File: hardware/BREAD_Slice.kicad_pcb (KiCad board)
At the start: 2 copper layers, 70 x 100 mm, 15 parts, among them J1 Conn_01x10_Female

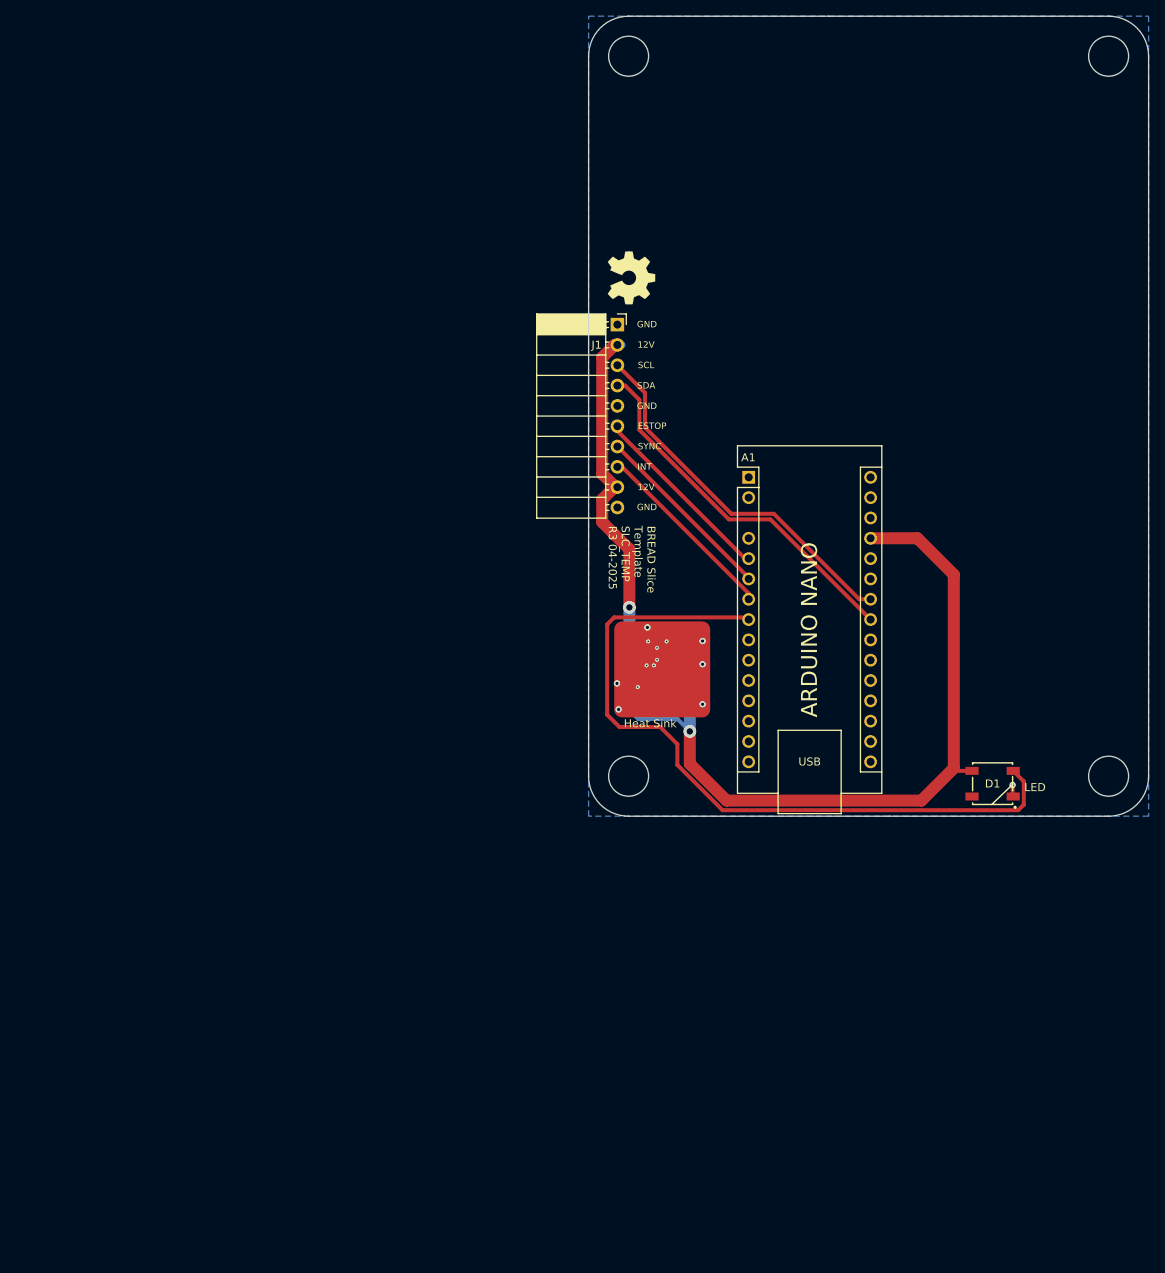
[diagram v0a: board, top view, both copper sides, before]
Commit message: final iteration of board with proper connectors and clean layout
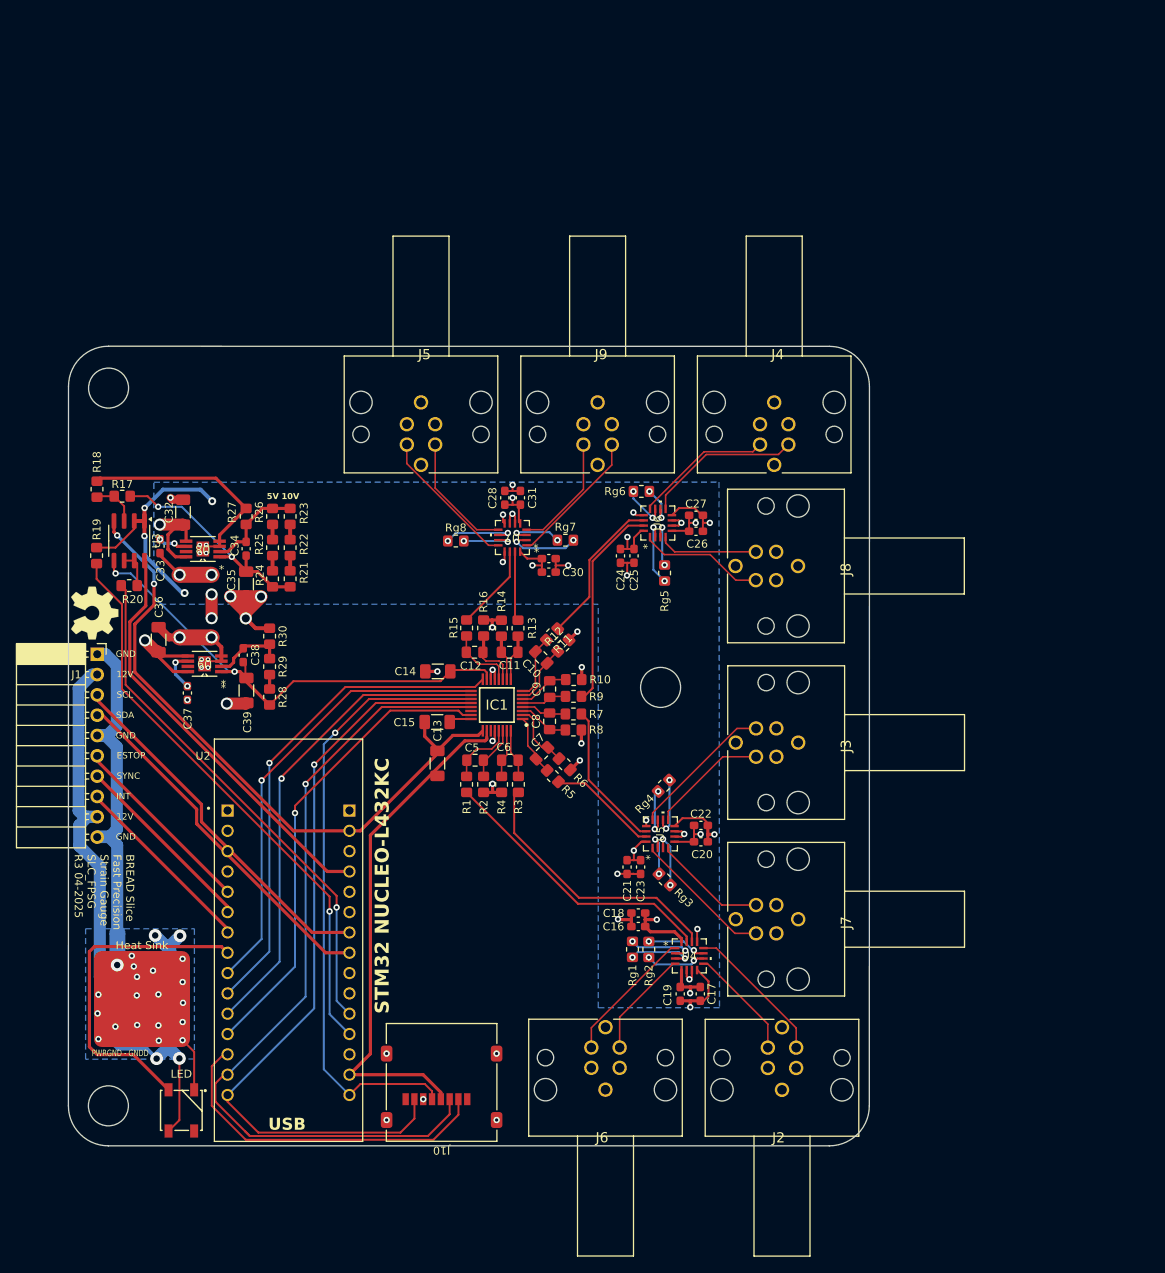
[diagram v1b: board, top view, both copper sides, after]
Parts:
- removed A1: Arduino_Nano_v3.x, Module:Arduino_Nano
- removed H4: MountingHole, MountingHole:MountingHole_5mm
- added C10: 10n, Capacitor_SMD:C_0805_2012Metric_Pad1.18x1.45mm_HandSolder, F.Cu at (116.7, 119.9)
- added C11: 10n, Capacitor_SMD:C_0805_2012Metric_Pad1.18x1.45mm_HandSolder, F.Cu at (112.7, 119.3)
- added C12: 10n, Capacitor_SMD:C_0805_2012Metric_Pad1.18x1.45mm_HandSolder, F.Cu at (108.4, 119.3)
- added C13: 1u, Capacitor_SMD:C_1206_3216Metric_Pad1.33x1.80mm_HandSolder, F.Cu at (103.7, 133.2)
- added C14: 1u, Capacitor_SMD:C_1206_3216Metric_Pad1.33x1.80mm_HandSolder, F.Cu at (103.8, 121.7)
- added C15: 220n, Capacitor_SMD:C_1206_3216Metric_Pad1.33x1.80mm_HandSolder, F.Cu at (103.7, 128.0)
- added C16: 1u, Capacitor_SMD:C_0603_1608Metric_Pad1.08x0.95mm_HandSolder, F.Cu at (128.8, 153.6)
- added C17: 10u, Capacitor_SMD:C_0603_1608Metric_Pad1.08x0.95mm_HandSolder, F.Cu at (136.6, 162.0)
- added C18: 1u, Capacitor_SMD:C_0603_1608Metric_Pad1.08x0.95mm_HandSolder, F.Cu at (128.8, 151.9)
- added C19: 10u, Capacitor_SMD:C_0603_1608Metric_Pad1.08x0.95mm_HandSolder, F.Cu at (134.1, 162.0)
- added C20: 1u, Capacitor_SMD:C_0603_1608Metric_Pad1.08x0.95mm_HandSolder, F.Cu at (136.6, 143.0)
- added C21: 10u, Capacitor_SMD:C_0603_1608Metric_Pad1.08x0.95mm_HandSolder, F.Cu at (127.4, 146.2)
- added C22: 1u, Capacitor_SMD:C_0603_1608Metric_Pad1.08x0.95mm_HandSolder, F.Cu at (136.6, 140.9)
- added C23: 10u, Capacitor_SMD:C_0603_1608Metric_Pad1.08x0.95mm_HandSolder, F.Cu at (129.1, 146.2)
- added C24: 1u, Capacitor_SMD:C_0603_1608Metric_Pad1.08x0.95mm_HandSolder, F.Cu at (126.6, 107.3)
- added C25: 10u, Capacitor_SMD:C_0603_1608Metric_Pad1.08x0.95mm_HandSolder, F.Cu at (128.3, 107.3)
- added C26: 1u, Capacitor_SMD:C_0603_1608Metric_Pad1.08x0.95mm_HandSolder, F.Cu at (136.0, 104.2)
- added C27: 10u, Capacitor_SMD:C_0603_1608Metric_Pad1.08x0.95mm_HandSolder, F.Cu at (136.0, 102.2)
- added C28: 1u, Capacitor_SMD:C_0603_1608Metric_Pad1.08x0.95mm_HandSolder, F.Cu at (112.1, 100.0)
- added C29: 10u, Capacitor_SMD:C_0603_1608Metric_Pad1.08x0.95mm_HandSolder, F.Cu at (117.6, 107.6)
- added C30: 1u, Capacitor_SMD:C_0603_1608Metric_Pad1.08x0.95mm_HandSolder, F.Cu at (117.6, 109.3)
- added C31: 10u, Capacitor_SMD:C_0603_1608Metric_Pad1.08x0.95mm_HandSolder, F.Cu at (114.1, 100.0)
- added C32: 10u X7R, Capacitor_SMD:C_1206_3216Metric_Pad1.33x1.80mm_HandSolder, F.Cu at (71.9, 101.8)
- added C33: 10n X7R, Capacitor_SMD:C_0603_1608Metric_Pad1.08x0.95mm_HandSolder, F.Cu at (69.0, 106.0)
- added C34: 10n X7R, Capacitor_SMD:C_0603_1608Metric_Pad1.08x0.95mm_HandSolder, F.Cu at (79.8, 106.4)
- added C35: 10u X7R, Capacitor_SMD:C_1206_3216Metric_Pad1.33x1.80mm_HandSolder, F.Cu at (79.8, 110.8)
- added C36: 10u X7R, Capacitor_SMD:C_1206_3216Metric_Pad1.33x1.80mm_HandSolder, F.Cu at (68.8, 117.7)
- added C37: 10n X7R, Capacitor_SMD:C_0603_1608Metric_Pad1.08x0.95mm_HandSolder, F.Cu at (72.5, 124.4)
- added C38: 10n X7R, Capacitor_SMD:C_0603_1608Metric_Pad1.08x0.95mm_HandSolder, F.Cu at (79.4, 119.7)
- added C39: 10u X7R, Capacitor_SMD:C_1206_3216Metric_Pad1.33x1.80mm_HandSolder, F.Cu at (79.8, 124.1)
- added C5: 10n, Capacitor_SMD:C_0805_2012Metric_Pad1.18x1.45mm_HandSolder, F.Cu at (108.4, 132.8)
- added C6: 10n, Capacitor_SMD:C_0805_2012Metric_Pad1.18x1.45mm_HandSolder, F.Cu at (112.8, 132.8)
- added C7: 10n, Capacitor_SMD:C_0805_2012Metric_Pad1.18x1.45mm_HandSolder, F.Cu at (116.8, 131.9)
- added C8: 10n, Capacitor_SMD:C_0805_2012Metric_Pad1.18x1.45mm_HandSolder, F.Cu at (117.7, 127.9)
- added C9: 10n, Capacitor_SMD:C_0805_2012Metric_Pad1.18x1.45mm_HandSolder, F.Cu at (117.7, 123.9)
- added IC1: ADS131M08IPBS, kml-custom:QFP50P700X700X120-32N, F.Cu at (111.1, 125.9)
- added J10: Micro_SD_Card, Connector_Card:microSD_HC_Molex_47219-2001, F.Cu at (104.2, 173.1)
- added J2: 1439890, kml-custom:1439890, F.Cu at (148.5, 168.7)
- added J3: 1439890, kml-custom:1439890, F.Cu at (143.5, 128.8)
- added J4: 1439890, kml-custom:1439890, F.Cu at (144.0, 93.3)
- added J5: 1439890, kml-custom:1439890, F.Cu at (99.9, 93.3)
- added J6: 1439890, kml-custom:1439890, F.Cu at (126.5, 168.7)
- added J7: 1439890, kml-custom:1439890, F.Cu at (143.5, 150.9)
- added J8: 1439890, kml-custom:1439890, F.Cu at (143.5, 106.8)
- added J9: 1439890, kml-custom:1439890, F.Cu at (122.0, 93.3)
- added NT1: NetTie_2, NetTie:NetTie-2_SMD_Pad2.0mm, B.Cu at (63.7, 156.4)
- added NT2: NetTie_2, NetTie:NetTie-2_SMD_Pad2.0mm, F.Cu at (73.5, 109.6)
- added NT3: NetTie_2, NetTie:NetTie-2_SMD_Pad2.0mm, F.Cu at (73.5, 117.5)
- added R1: 1k, Resistor_SMD:R_0805_2012Metric_Pad1.20x1.40mm_HandSolder, F.Cu at (107.3, 135.8)
- added R10: 1k, Resistor_SMD:R_0805_2012Metric_Pad1.20x1.40mm_HandSolder, F.Cu at (120.7, 122.7)
- added R11: 1k, Resistor_SMD:R_0805_2012Metric_Pad1.20x1.40mm_HandSolder, F.Cu at (118.0, 117.1)
- added R12: 1k, Resistor_SMD:R_0805_2012Metric_Pad1.20x1.40mm_HandSolder, F.Cu at (119.5, 118.5)
- added R13: 1k, Resistor_SMD:R_0805_2012Metric_Pad1.20x1.40mm_HandSolder, F.Cu at (113.8, 116.3)
- added R14: 1k, Resistor_SMD:R_0805_2012Metric_Pad1.20x1.40mm_HandSolder, F.Cu at (111.7, 116.3)
- added R15: 1k, Resistor_SMD:R_0805_2012Metric_Pad1.20x1.40mm_HandSolder, F.Cu at (107.3, 116.3)
- added R16: 1k, Resistor_SMD:R_0805_2012Metric_Pad1.20x1.40mm_HandSolder, F.Cu at (109.5, 116.3)
- added R17: 50k 1%, Resistor_SMD:R_0805_2012Metric_Pad1.20x1.40mm_HandSolder, F.Cu at (64.3, 99.8)
- added R18: 50k 1%, Resistor_SMD:R_0805_2012Metric_Pad1.20x1.40mm_HandSolder, F.Cu at (61.1, 98.9)
- added R19: 1k, Resistor_SMD:R_0805_2012Metric_Pad1.20x1.40mm_HandSolder, F.Cu at (61.1, 107.2)
- added R2: 1k, Resistor_SMD:R_0805_2012Metric_Pad1.20x1.40mm_HandSolder, F.Cu at (109.5, 135.8)
- added R20: 1k, Resistor_SMD:R_0805_2012Metric_Pad1.20x1.40mm_HandSolder, F.Cu at (65.2, 111.0)
- added R21: 680 1%, Resistor_SMD:R_0805_2012Metric_Pad1.20x1.40mm_HandSolder, F.Cu at (85.3, 110.1)
- added R22: 680k 1%, Resistor_SMD:R_0805_2012Metric_Pad1.20x1.40mm_HandSolder, F.Cu at (85.3, 106.2)
- added R23: 63.4k 1%, Resistor_SMD:R_0805_2012Metric_Pad1.20x1.40mm_HandSolder, F.Cu at (85.3, 102.3)
- added R24: 100 1%, Resistor_SMD:R_0805_2012Metric_Pad1.20x1.40mm_HandSolder, F.Cu at (83.1, 110.1)
- added R25: 300k 1%, Resistor_SMD:R_0805_2012Metric_Pad1.20x1.40mm_HandSolder, F.Cu at (83.1, 106.2)
- added R26: 71.5k 1%, Resistor_SMD:R_0805_2012Metric_Pad1.20x1.40mm_HandSolder, F.Cu at (83.1, 102.3)
- added R27: 100k 1%, Resistor_SMD:R_0805_2012Metric_Pad1.20x1.40mm_HandSolder, F.Cu at (79.8, 102.3)
- added R28: 300k 1%, Resistor_SMD:R_0805_2012Metric_Pad1.20x1.40mm_HandSolder, F.Cu at (82.7, 124.9)
- added R29: 71.5k 1%, Resistor_SMD:R_0805_2012Metric_Pad1.20x1.40mm_HandSolder, F.Cu at (82.7, 121.1)
- added R3: 1k, Resistor_SMD:R_0805_2012Metric_Pad1.20x1.40mm_HandSolder, F.Cu at (113.8, 135.8)
- added R30: 100k 1%, Resistor_SMD:R_0805_2012Metric_Pad1.20x1.40mm_HandSolder, F.Cu at (82.7, 117.3)
- added R4: 1k, Resistor_SMD:R_0805_2012Metric_Pad1.20x1.40mm_HandSolder, F.Cu at (111.7, 135.8)
- added R5: 1k, Resistor_SMD:R_0805_2012Metric_Pad1.20x1.40mm_HandSolder, F.Cu at (118.1, 134.8)
- added R6: 1k, Resistor_SMD:R_0805_2012Metric_Pad1.20x1.40mm_HandSolder, F.Cu at (119.6, 133.3)
- added R7: 1k, Resistor_SMD:R_0805_2012Metric_Pad1.20x1.40mm_HandSolder, F.Cu at (120.7, 127.0)
- added R8: 1k, Resistor_SMD:R_0805_2012Metric_Pad1.20x1.40mm_HandSolder, F.Cu at (120.7, 129.0)
- added R9: 1k, Resistor_SMD:R_0805_2012Metric_Pad1.20x1.40mm_HandSolder, F.Cu at (120.7, 124.8)
- added Rg1: -, Resistor_SMD:R_0805_2012Metric_Pad1.20x1.40mm_HandSolder, F.Cu at (128.1, 156.4)
- added Rg2: -, Resistor_SMD:R_0805_2012Metric_Pad1.20x1.40mm_HandSolder, F.Cu at (130.1, 156.4)
- added Rg3: -, Resistor_SMD:R_0805_2012Metric_Pad1.20x1.40mm_HandSolder, F.Cu at (132.1, 147.7)
- added Rg4: -, Resistor_SMD:R_0805_2012Metric_Pad1.20x1.40mm_HandSolder, F.Cu at (132.0, 136.0)
- added Rg5: -, Resistor_SMD:R_0805_2012Metric_Pad1.20x1.40mm_HandSolder, F.Cu at (132.1, 109.4)
- added Rg6: -, Resistor_SMD:R_0805_2012Metric_Pad1.20x1.40mm_HandSolder, F.Cu at (129.2, 99.2)
- added Rg7: -, Resistor_SMD:R_0805_2012Metric_Pad1.20x1.40mm_HandSolder, F.Cu at (119.7, 105.3)
- added Rg8: -, Resistor_SMD:R_0805_2012Metric_Pad1.20x1.40mm_HandSolder, F.Cu at (106.0, 105.4)
- added U2: NUCLEO-L432KC, kml-custom:MODULE_NUCLEO-L432KC, F.Cu at (85.1, 155.3)
- added U3: MCP6022, Package_SO:SOIC-8_3.9x4.9mm_P1.27mm, F.Cu at (65.2, 105.4)
- added U4: AD8426BCPZ-WP, kml-custom:CP_16_19_ADI, F.Cu at (135.2, 157.3)
- added U5: AD8426BCPZ-WP, kml-custom:CP_16_19_ADI, F.Cu at (131.6, 142.0)
- added U6: AD8426BCPZ-WP, kml-custom:CP_16_19_ADI, F.Cu at (131.2, 103.2)
- added U7: AD8426BCPZ-WP, kml-custom:CP_16_19_ADI, F.Cu at (113.1, 105.0)
- added U8: TPS7A4901DGNR, kml-custom:DGN8_1P89X1P57, F.Cu at (74.4, 106.4)
- added U9: TPS7A4901DGNR, kml-custom:DGN8_1P89X1P57, F.Cu at (74.6, 120.8)
- HS1: footprint KML-Custom:Thermal Pad -> kml-custom:Thermal Pad
- U1: value ~ -> AP63205
- moved D1 109.3 mm to (71.7, 176.6), turned to 90 degrees
- moved H3 96.8 mm to (131.6, 123.7)
- moved Logo1 79.1 mm to (60.9, 114.4)
- moved H1 77.1 mm to (62.6, 86.3)
- moved C1 77.0 mm to (63.8, 160.7)
- moved C2 77.0 mm to (66.1, 167.5)
- moved J1 77.0 mm to (61.2, 119.6)
- moved L1 77.0 mm to (68.8, 164.0)
- moved U1 77.0 mm to (63.7, 164.0)
- moved C3 77.0 mm to (68.8, 160.7)
- moved HS1 77.0 mm to (66.8, 162.7)
- moved H2 77.0 mm to (62.6, 176.0)
- moved C4 77.0 mm to (68.8, 157.6)
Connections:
- net +5V renamed +5VD
- C1 pad 1: GND -> GNDD
- C3 pad 1: GND -> GNDD
- C4 pad 1: GND -> GNDD
- D1 pad 3: GND -> GNDD
- HS1 pad 1: GND -> GNDD
- J1 pad 1: GND -> GNDPWR
- J1 pad 10: GND -> GNDPWR
- J1 pad 5: GND -> GNDPWR
- J1 pad 6: /E_STOP -> /ESTOP
- U1 pad 4: GND -> GNDD
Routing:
- net GNDA: track 0.00 -> 119.3 mm, vias 0 -> 38
- net GNDD: track 0.00 -> 108.5 mm, vias 0 -> 26
- net /MOSI: track 0.00 -> 104.2 mm, vias 0 -> 1
- net /MISO: track 0.00 -> 97.5 mm, vias 0 -> 1
- net /SCK: track 0.00 -> 78.2 mm, vias 0 -> 1
- net VAA: track 0.00 -> 75.0 mm, vias 0 -> 10
- net /VMID_SENS: track 0.00 -> 71.9 mm, vias 0 -> 1
- net /VADC_SENS: track 0.00 -> 65.3 mm, vias 0 -> 1
- net +3V3: track 0.00 -> 64.8 mm
- net /RST_ADC: track 0.00 -> 62.0 mm, vias 0 -> 1
- net +3.3VADC: track 0.00 -> 61.8 mm, vias 0 -> 2
- net /DRDY: track 0.00 -> 60.5 mm, vias 0 -> 1
- net /CLK_MCO: track 0.00 -> 59.2 mm, vias 0 -> 1
- net /ADC_CS: track 0.00 -> 56.7 mm, vias 0 -> 1
- net GNDPWR: track 0.00 -> 52.2 mm, vias 0 -> 4
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- added copper zone on In2.Cu, net +12V
- added copper zone on In2.Cu, net +3.3VADC
- added copper zone on In2.Cu, net +5VD
- added copper zone on B.Cu, net /VMID
- added copper zone on In1.Cu, net GNDA
- added copper zone on B.Cu, net GNDD
- added copper zone on In1.Cu, net GNDD
- added copper zone on In1.Cu, net GNDPWR
- added copper zone on In2.Cu, net VAA
- removed copper zone on B.Cu, net GND
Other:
- board size 70 x 100 mm -> 100.1 x 100 mm
- copper layers 2 -> 4
- board text added: "10V"
- board text added: "12V->5V Sw.Reg"
- board text added: "5V"
- board text added: "BREAD Slice Fast Precision Strain Gauge SLC_FPSG R3 04-2025"
- board text added: "PWRGND - GNDD"
- board text added: "STM32 NUCLEO-L432KC"
- board text added: "USB"
- board text removed: "12V->5V Reg"
- board text removed: "ARDUINO NANO"
- board text removed: "BREAD Slice Template SLC_TEMP R3 04-2025"
